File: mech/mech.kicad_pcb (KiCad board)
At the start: 2 copper layers, 66 x 120.7 mm, 54 parts, among them P1 Pump_Motor_DC, P2 Pump_Motor_DC, T1 DS18B20, T2 DS18B20, U1 DHT22, U2 PCA9685PW, U3 ADC128D818, U4 ADC128D818

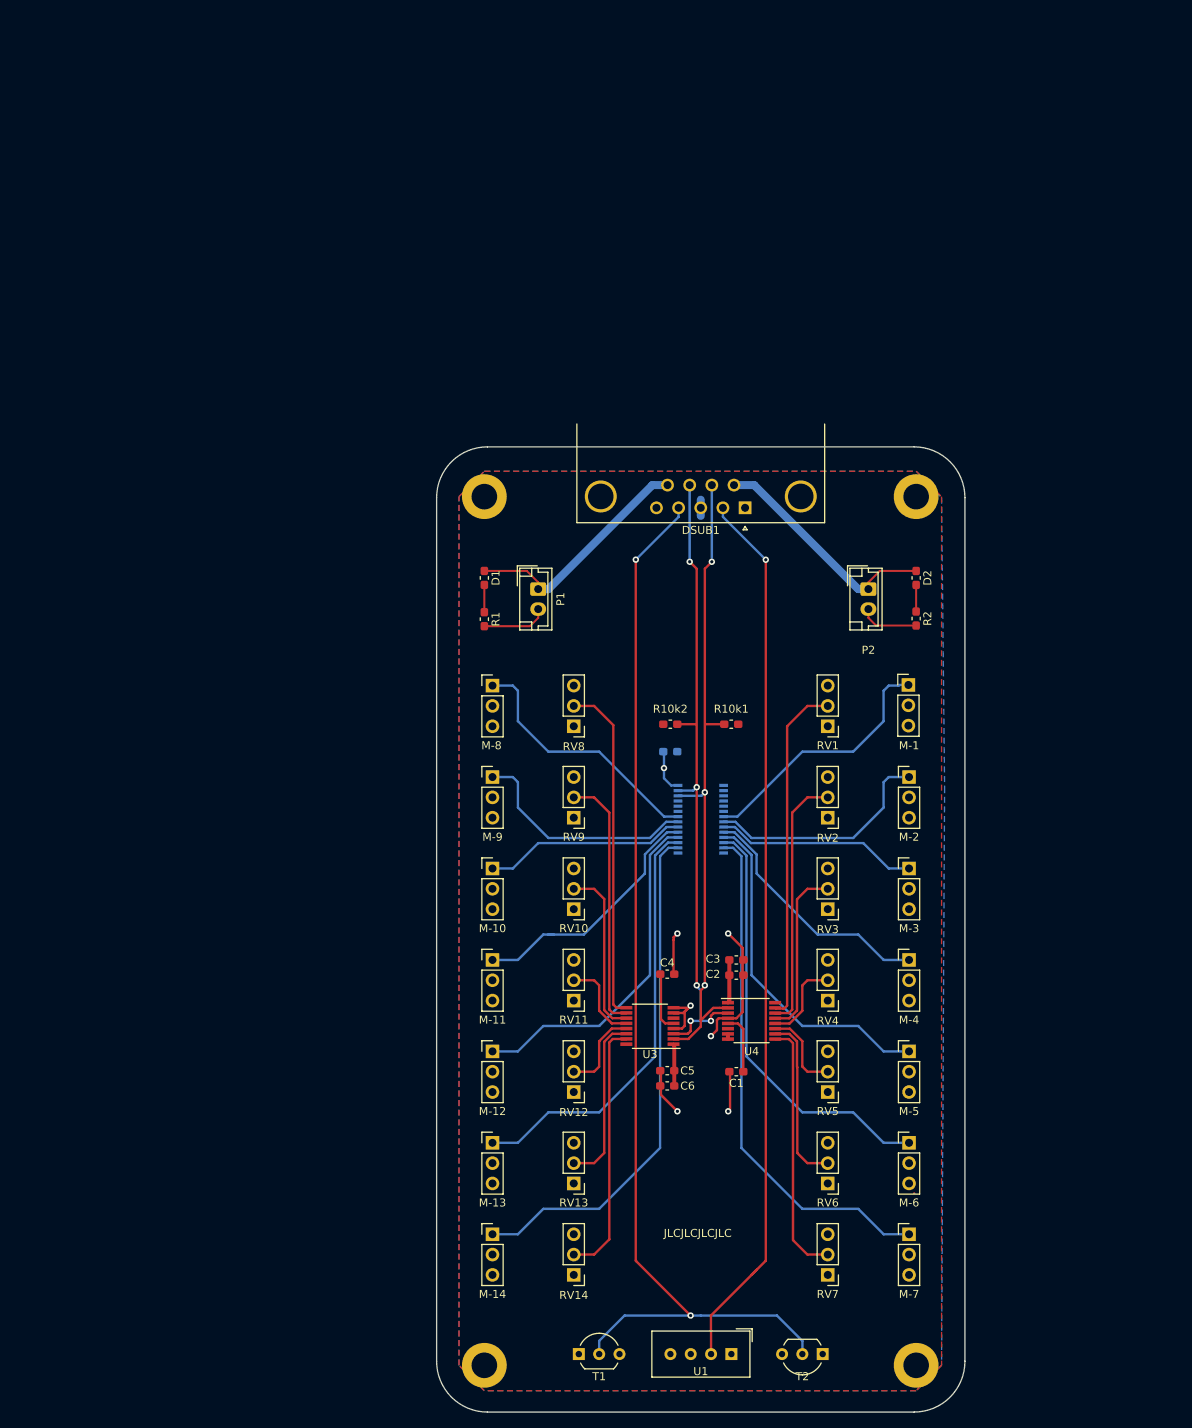
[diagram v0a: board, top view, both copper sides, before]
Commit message: WIP sensor PCB - delete files
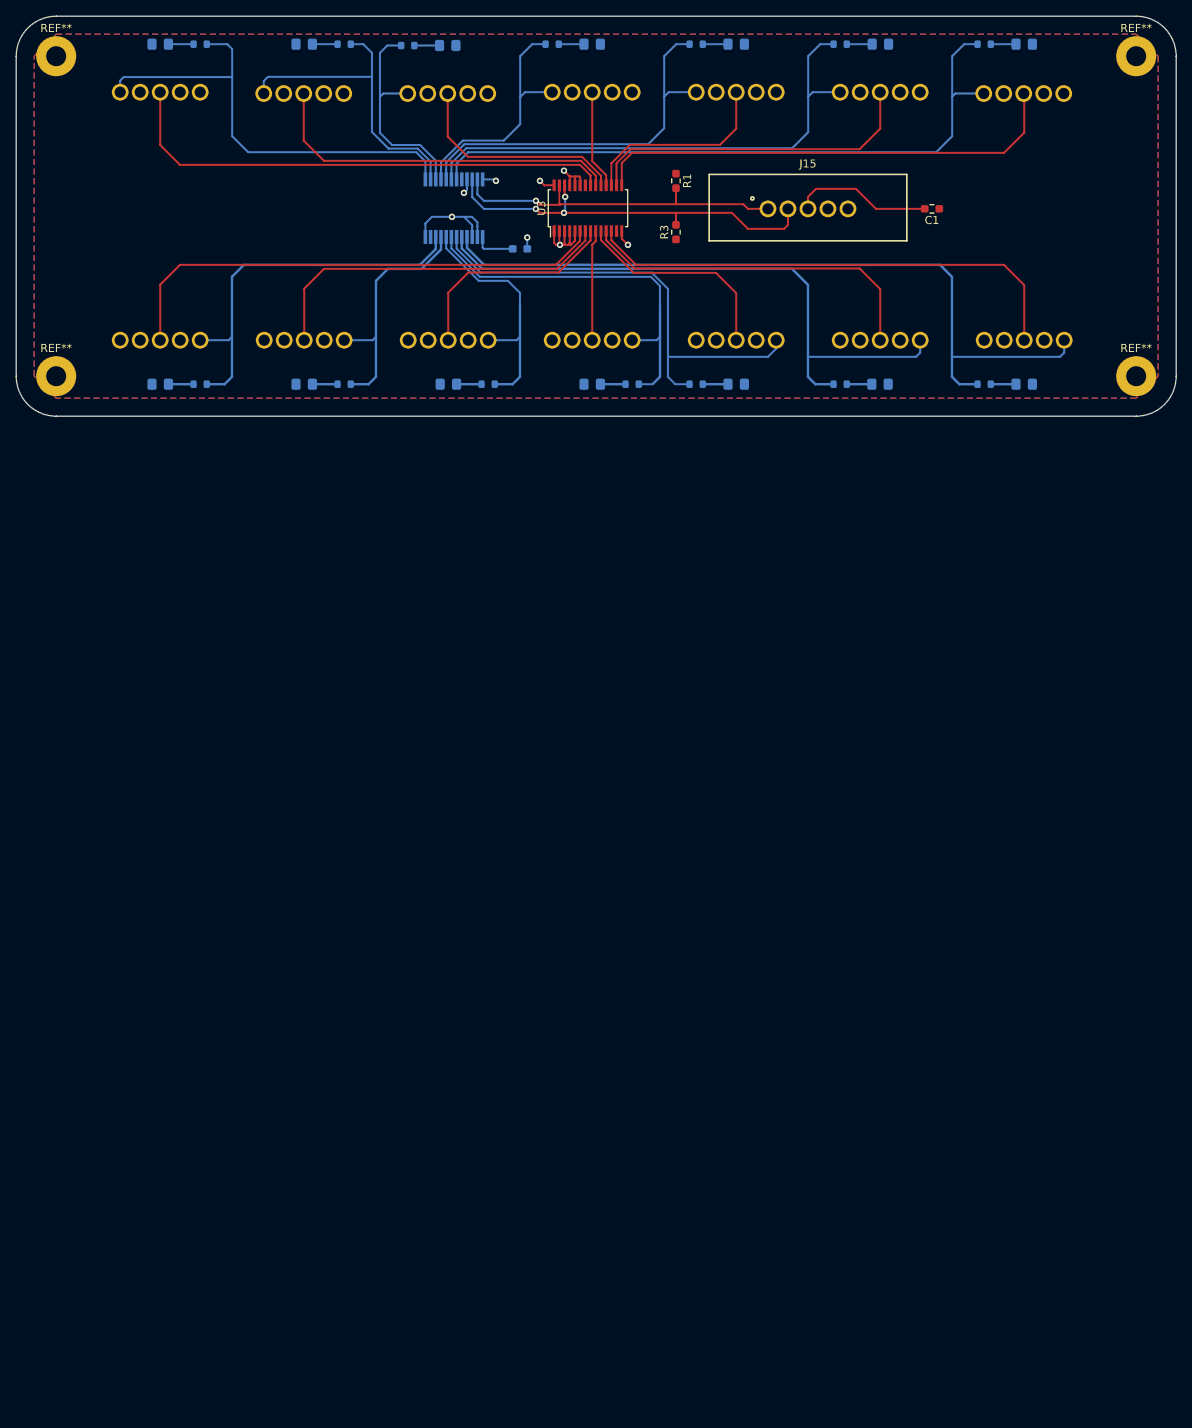
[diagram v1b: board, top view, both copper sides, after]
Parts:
- removed  : MountingHole_3.2mm_M3_DIN965_Pad, MountingHole:MountingHole_3.2mm_M3_DIN965_Pad (x4)
- removed C0, C4, C6: C100nF, Resistor_SMD:R_0603_1608Metric_Pad1.05x0.95mm_HandSolder
- removed C2: 10nF, Resistor_SMD:R_0603_1608Metric_Pad1.05x0.95mm_HandSolder
- removed C3: 100nF, Resistor_SMD:R_0603_1608Metric_Pad1.05x0.95mm_HandSolder
- removed C5: C10nF, Resistor_SMD:R_0603_1608Metric_Pad1.05x0.95mm_HandSolder
- removed DSUB1: DB9_Male, Connector_Dsub:DSUB-9_Male_Horizontal_P2.77x2.84mm_EdgePinOffset7.70mm_Housed_MountingHolesOffset9.12mm
- removed M-1, M-10, M-11, M-12, M-13, M-14, M-2, M-3, M-4, M-5, M-6, M-7, M-8, M-9: Motor_Servo_Hitec, Connector_PinHeader_2.54mm:PinHeader_1x03_P2.54mm_Vertical
- removed P1, P2: Pump_Motor_DC, Connector_JST:JST_EH_B2B-EH-A_1x02_P2.50mm_Vertical
- removed R10k1, R10k2: R, Resistor_SMD:R_0603_1608Metric_Pad1.05x0.95mm_HandSolder
- removed RV1, RV10, RV11, RV12, RV13, RV14, RV2, RV3, RV4, RV5, RV6, RV7, RV8, RV9: R_POT, Connector_PinHeader_2.54mm:PinHeader_1x03_P2.54mm_Vertical
- removed T1, T2: DS18B20, Package_TO_SOT_THT:TO-92_Inline_Wide
- removed U1: DHT22, Sensor:Aosong_DHT11_5.5x12.0_P2.54mm
- removed U4: ADC128D818, Package_SO:TSSOP-16_4.4x5mm_P0.65mm
- added D10: LED, LED_SMD:LED_0805_2012Metric_Pad1.15x1.40mm_HandSolder, B.Cu at (70.0, 45.1)
- added D11: LED, LED_SMD:LED_0805_2012Metric_Pad1.15x1.40mm_HandSolder, B.Cu at (88.0, 44.9)
- added D12: LED, LED_SMD:LED_0805_2012Metric_Pad1.15x1.40mm_HandSolder, B.Cu at (106.0, 44.9)
- added D13: LED, LED_SMD:LED_0805_2012Metric_Pad1.15x1.40mm_HandSolder, B.Cu at (124.1, 44.9)
- added D14: LED, LED_SMD:LED_0805_2012Metric_Pad1.15x1.40mm_HandSolder, B.Cu at (142.0, 44.9)
- added D3: LED, LED_SMD:LED_0805_2012Metric_Pad1.15x1.40mm_HandSolder, B.Cu at (70.1, 87.4)
- added D4: LED, LED_SMD:LED_0805_2012Metric_Pad1.15x1.40mm_HandSolder, B.Cu at (88.0, 87.4)
- added D5: LED, LED_SMD:LED_0805_2012Metric_Pad1.15x1.40mm_HandSolder, B.Cu at (106.0, 87.4)
- added D6: LED, LED_SMD:LED_0805_2012Metric_Pad1.15x1.40mm_HandSolder, B.Cu at (124.0, 87.4)
- added D7: LED, LED_SMD:LED_0805_2012Metric_Pad1.15x1.40mm_HandSolder, B.Cu at (142.0, 87.4)
- added D8: LED, LED_SMD:LED_0805_2012Metric_Pad1.15x1.40mm_HandSolder, B.Cu at (34.0, 44.9)
- added D9: LED, LED_SMD:LED_0805_2012Metric_Pad1.15x1.40mm_HandSolder, B.Cu at (52.0, 44.9)
- added J1: Conn_01x05_Female, Stardust:691382000005, B.Cu at (34.0, 81.9)
- added J10: Conn_01x05_Female, Stardust:691382000005, B.Cu at (70.0, 51.1)
- added J11: Conn_01x05_Female, Stardust:691382000005, B.Cu at (88.0, 50.9)
- added J12: Conn_01x05_Female, Stardust:691382000005, B.Cu at (106.0, 50.9)
- added J13: Conn_01x05_Female, Stardust:691382000005, B.Cu at (124.0, 50.9)
- added J14: Conn_01x05_Female, Stardust:691382000005, B.Cu at (142.0, 51.1)
- added J15: Conn_01x05_Female, Stardust:691382030005, F.Cu at (115.0, 65.5)
- added J2: Conn_01x05_Female, Stardust:691382000005, B.Cu at (52.0, 81.9)
- added J3: Conn_01x05_Female, Stardust:691382000005, B.Cu at (70.0, 81.9)
- added J4: Conn_01x05_Female, Stardust:691382000005, B.Cu at (88.0, 81.9)
- added J5: Conn_01x05_Female, Stardust:691382000005, B.Cu at (106.0, 81.9)
- added J6: Conn_01x05_Female, Stardust:691382000005, B.Cu at (124.0, 81.9)
- added J7: Conn_01x05_Female, Stardust:691382000005, B.Cu at (142.0, 81.9)
- added J8: Conn_01x05_Female, Stardust:691382000005, B.Cu at (34.0, 50.9)
- added J9: Conn_01x05_Female, Stardust:691382000005, B.Cu at (52.0, 51.1)
- added R10: R330, Resistor_SMD:R_0603_1608Metric, B.Cu at (119.0, 87.4)
- added R11: R330, Resistor_SMD:R_0603_1608Metric, B.Cu at (137.0, 87.4)
- added R12: R330, Resistor_SMD:R_0603_1608Metric, B.Cu at (39.0, 44.9)
- added R13: R330, Resistor_SMD:R_0603_1608Metric, B.Cu at (57.0, 44.9)
- added R14: R330, Resistor_SMD:R_0603_1608Metric, B.Cu at (65.0, 45.1)
- added R15: R330, Resistor_SMD:R_0603_1608Metric, B.Cu at (83.0, 44.9)
- added R16: R330, Resistor_SMD:R_0603_1608Metric, B.Cu at (101.0, 44.9)
- added R17: R330, Resistor_SMD:R_0603_1608Metric, B.Cu at (119.0, 44.9)
- added R18: R330, Resistor_SMD:R_0603_1608Metric, B.Cu at (137.0, 44.9)
- added R3: R10k, Resistor_SMD:R_0603_1608Metric_Pad0.98x0.95mm_HandSolder, F.Cu at (98.5, 68.4)
- added R5: R330, Resistor_SMD:R_0603_1608Metric, B.Cu at (39.0, 87.4)
- added R6: R330, Resistor_SMD:R_0603_1608Metric, B.Cu at (57.0, 87.4)
- added R7: R330, Resistor_SMD:R_0603_1608Metric, B.Cu at (75.0, 87.4)
- added R8: R330, Resistor_SMD:R_0603_1608Metric, B.Cu at (93.0, 87.4)
- added R9: R330, Resistor_SMD:R_0603_1608Metric, B.Cu at (101.0, 87.4)
- added REF**: MountingHole_2.5mm_Pad, MountingHole:MountingHole_2.5mm_Pad, F.Cu at (21.0, 86.4)
- added REF**: MountingHole_2.5mm_Pad, MountingHole:MountingHole_2.5mm_Pad, F.Cu at (21.0, 46.4)
- added REF**: MountingHole_2.5mm_Pad, MountingHole:MountingHole_2.5mm_Pad, F.Cu at (156.0, 86.4)
- added REF**: MountingHole_2.5mm_Pad, MountingHole:MountingHole_2.5mm_Pad, F.Cu at (156.0, 46.4)
- C1: footprint Resistor_SMD:R_0603_1608Metric_Pad1.05x0.95mm_HandSolder -> Resistor_SMD:R_0603_1608Metric_Pad0.98x0.95mm_HandSolder
- D1, D2: footprint Resistor_SMD:R_0603_1608Metric_Pad1.05x0.95mm_HandSolder -> LED_SMD:LED_0805_2012Metric_Pad1.15x1.40mm_HandSolder; moved to B.Cu
- R1: value 1k -> R10k; footprint Resistor_SMD:R_0603_1608Metric_Pad1.05x0.95mm_HandSolder -> Resistor_SMD:R_0603_1608Metric_Pad0.98x0.95mm_HandSolder
- R2: value 1k -> R10k; footprint Resistor_SMD:R_0603_1608Metric_Pad1.05x0.95mm_HandSolder -> Resistor_SMD:R_0603_1608Metric_Pad0.98x0.95mm_HandSolder; moved to B.Cu
- U2: value PCA9685PW -> TCA9555DBR; footprint Package_SO:TSSOP-28_4.4x9.7mm_P0.65mm -> Package_SO:SSOP-24_5.3x8.2mm_P0.65mm
- U3: value ADC128D818 -> PCA9685PW; footprint Package_SO:TSSOP-16_4.4x5mm_P0.65mm -> Package_SO:TSSOP-28_4.4x9.7mm_P0.65mm
- moved C1 110.6 mm to (130.5, 65.5)
- moved U3 102.5 mm to (87.5, 65.4), turned to 90 degrees
- moved U2 82.4 mm to (70.8, 65.4), turned to 90 degrees
- moved D2 80.2 mm to (52.0, 87.4), turned to 0 degrees
- moved R2 67.7 mm to (79.0, 70.5), turned to 180 degrees
- moved R1 59.8 mm to (98.5, 62.0)
- moved D1 47.2 mm to (34.0, 87.4), turned to 0 degrees
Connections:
- D1 pad 1: +12V -> GND
- D2 pad 1: +12V -> GND
- R1 pad 1: Net-(D1-Pad2) -> +5V
- R1 pad 2: GND -> I2C-SDA
- R2 pad 1: Net-(D2-Pad2) -> +5V
- R2 pad 2: GND -> Net-(R2-Pad2)
- U2 pad 1: GND -> Net-(R2-Pad2)
- U2 pad 10: Net-(M-4-Pad1) -> SW-1
- U2 pad 11: Net-(M-5-Pad1) -> (no net)
- U2 pad 12: Net-(M-6-Pad1) -> GND
- U2 pad 13: Net-(M-7-Pad1) -> SW-8
- U2 pad 14: GND -> SW-9
- U2 pad 15: Net-(U2-Pad15) -> SW-10
- U2 pad 16: Net-(M-14-Pad1) -> SW-11
- U2 pad 17: Net-(M-13-Pad1) -> SW-12
- U2 pad 18: Net-(M-12-Pad1) -> SW-13
- U2 pad 19: Net-(M-11-Pad1) -> SW-14
- U2 pad 20: Net-(M-10-Pad1) -> (no net)
- U2 pad 21: Net-(M-9-Pad1) -> GND
- U2 pad 22: Net-(M-8-Pad1) -> I2C-SCL
- U2 pad 23: GND -> I2C-SDA
- U2 pad 24: GND -> +5V
- U2 pad 4: GND -> SW-7
- U2 pad 5: GND -> SW-6
- U2 pad 6: Net-(U2-Pad6) -> SW-5
- U2 pad 7: Net-(M-1-Pad1) -> SW-4
- U2 pad 8: Net-(M-2-Pad1) -> SW-3
- U2 pad 9: Net-(M-3-Pad1) -> SW-2
- U3 pad 1: +5V -> GND
- U3 pad 10: Net-(RV9-Pad2) -> PWM-5
- U3 pad 11: Net-(RV10-Pad2) -> PWM-6
- U3 pad 12: Net-(RV11-Pad2) -> PWM-7
- U3 pad 13: Net-(RV12-Pad2) -> (no net)
- U3 pad 14: Net-(RV13-Pad2) -> GND
- U3 pad 15: Net-(RV14-Pad2) -> PWM-14
- U3 pad 16: Net-(U3-Pad16) -> PWM-13
- U3 pad 2: I2C-SCL -> GND
- U3 pad 3: I2C-SDA -> GND
- U3 pad 5: +5V -> GND
- U3 pad 6: Net-(U3-Pad6) -> PWM-1
- U3 pad 7: GND -> PWM-2
- U3 pad 8: GND -> PWM-3
- U3 pad 9: Net-(RV8-Pad2) -> PWM-4
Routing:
- net 1Wire: track 137.3 -> 0.00 mm, vias 2 -> 0
- net DHT22: track 111.7 -> 0.00 mm, vias 1 -> 0
- net SW-7: track 0.00 -> 95.4 mm
- net SW-14: track 0.00 -> 83.3 mm
- net SW-6: track 0.00 -> 77.5 mm
- net SW-13: track 0.00 -> 65.8 mm
- net Net-(M-7-Pad1): track 64.6 -> 0.00 mm
- net Net-(M-14-Pad1): track 64.6 -> 0.00 mm
- net PWM-8: track 0.00 -> 63.2 mm
- net PWM-1: track 0.00 -> 62.9 mm
- net PWM-7: track 0.00 -> 62.0 mm
- net PWM-14: track 0.00 -> 59.7 mm
- net +12V: track 59.3 -> 0.00 mm
- net SW-5: track 0.00 -> 59.0 mm
- net SW-8: track 0.00 -> 57.7 mm
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- added copper zone on In2.Cu, net +5P
- added copper zone on In1.Cu, net GND
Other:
- board size 66 x 120.7 mm -> 145 x 50 mm
- copper layers 2 -> 4
- board text removed: "JLCJLCJLCJLC"
- board text removed: "Stardust 2020"
- board text removed: "contact@yasiu.pl"
